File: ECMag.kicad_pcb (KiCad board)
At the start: 2 copper layers, 48 parts, among them J1 Conn_01x12, J2 Conn_01x05, J3 Conn_01x04, J4 USB_B, J5 Barrel_Jack_SW, J6 Conn_01x04, K1 Tactil Switch NA, K2 Tactil Switch B3F NA, K3 Tactil Switch NA, K4 Tactil Switch NA, P1 25K, Q1 BC548, U1 ATmega328P-PU, U2 PIC18F2550-ISO, U3 LM2577, Y1 16MHz, Y2 20MHz

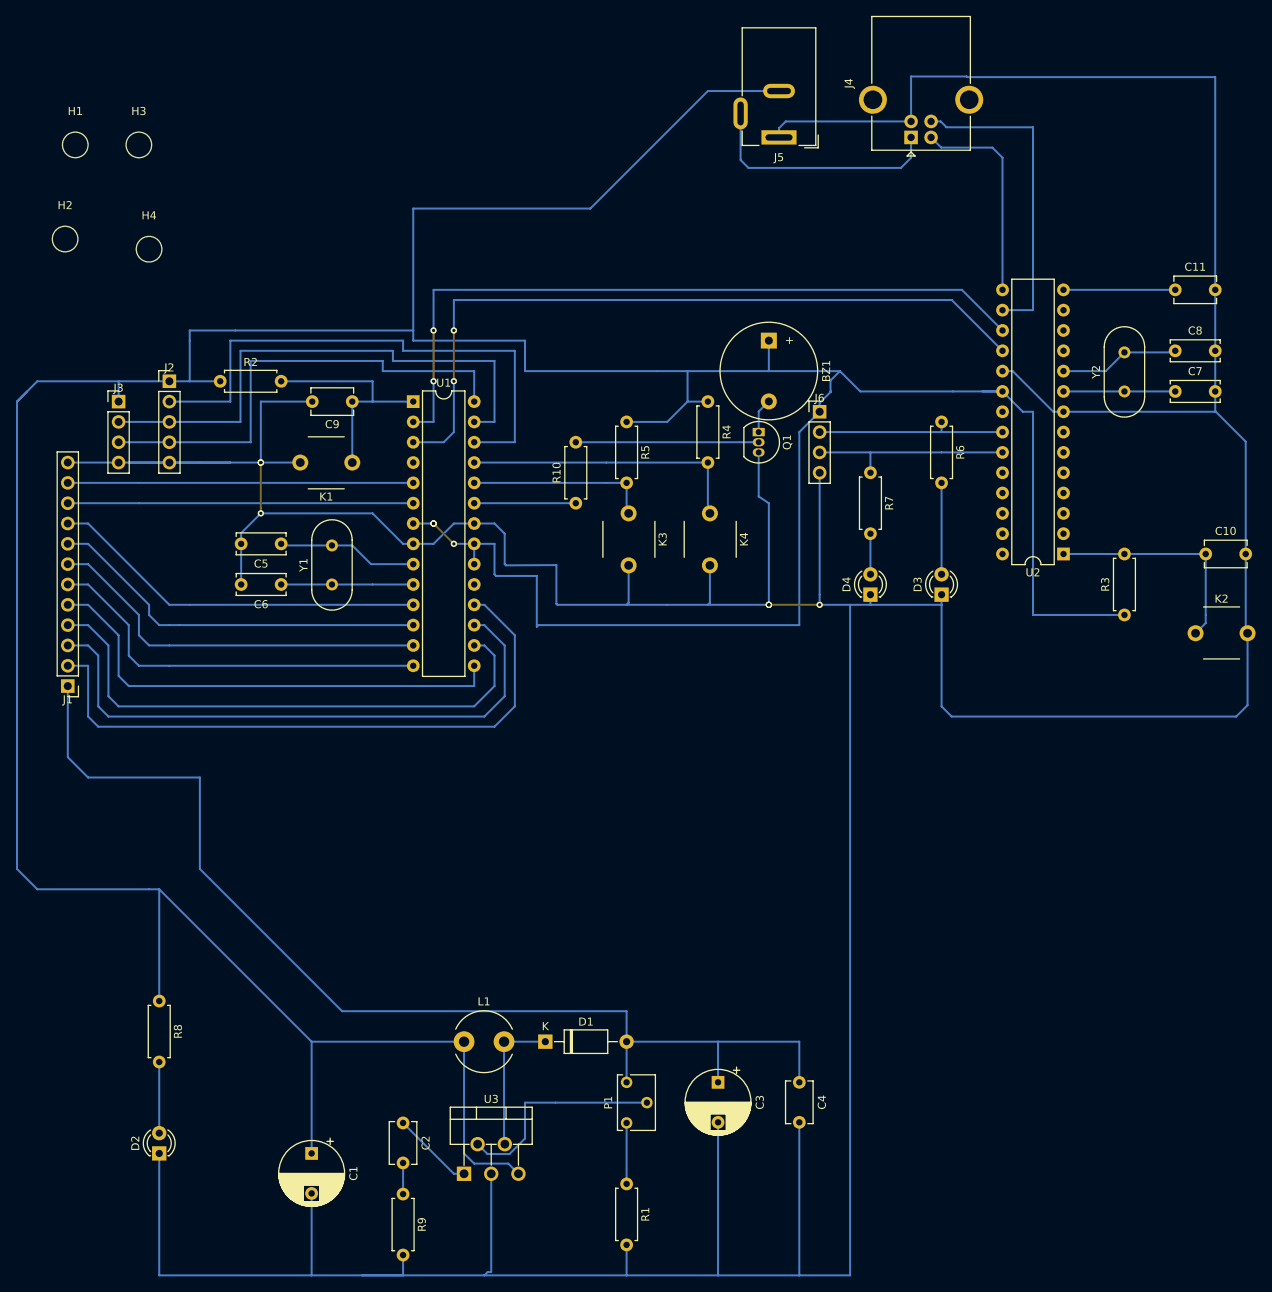
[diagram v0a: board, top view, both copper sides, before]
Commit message: primera versión del pcb
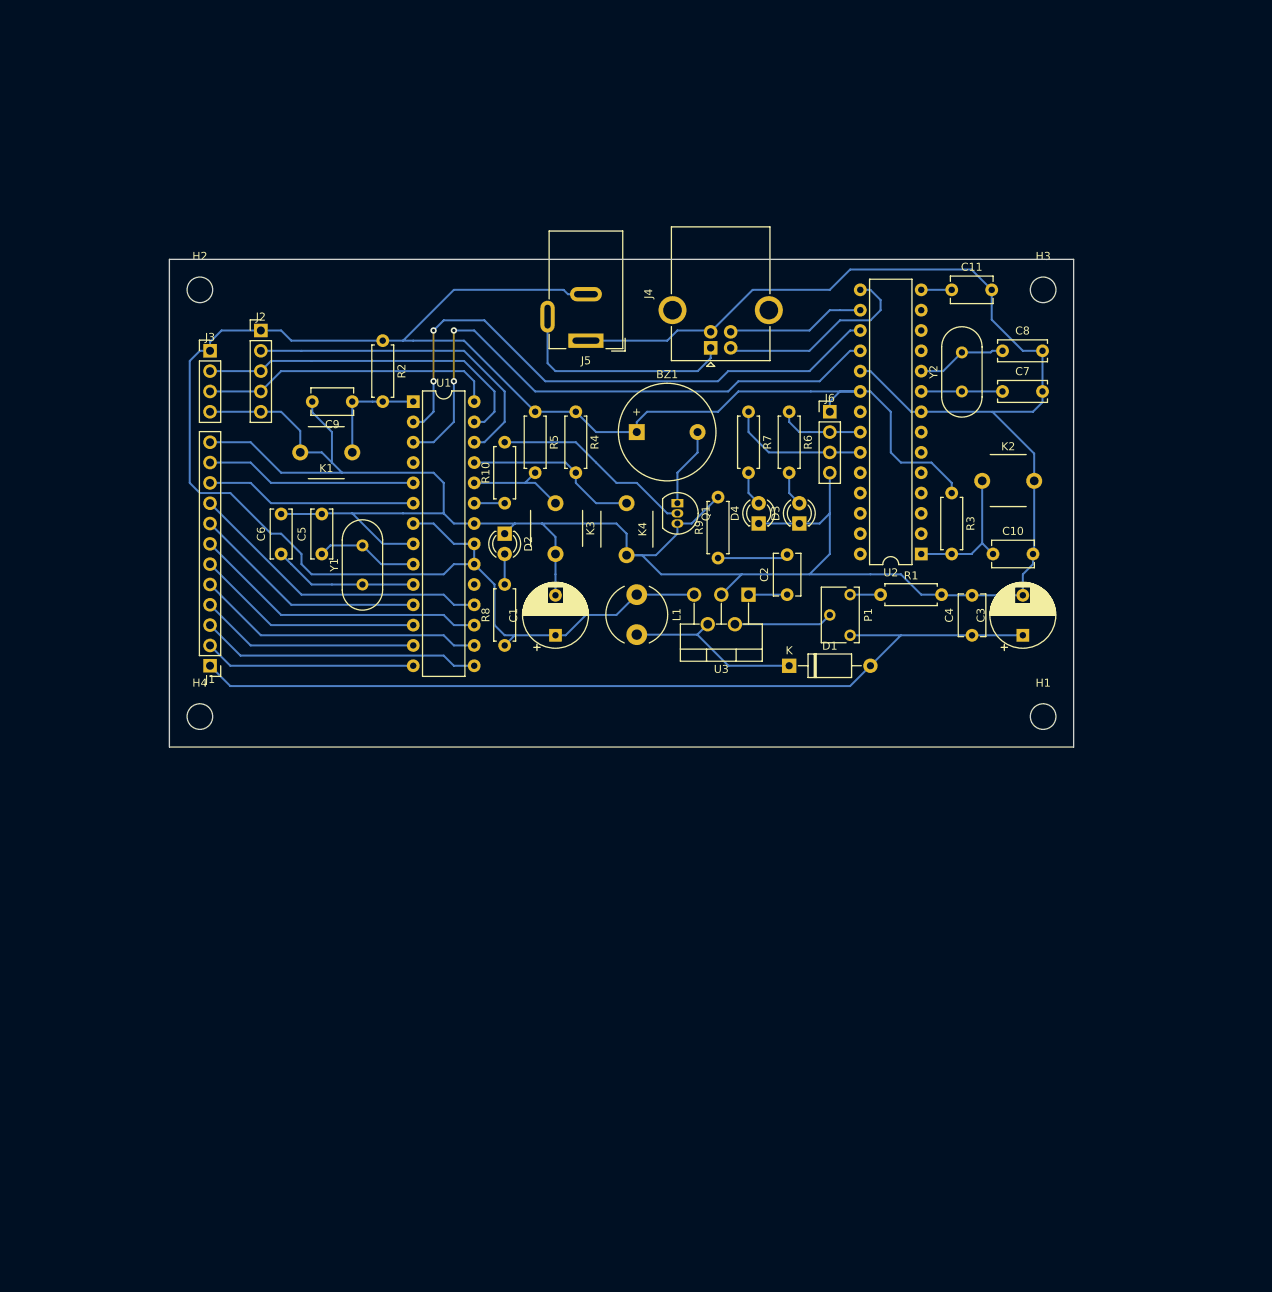
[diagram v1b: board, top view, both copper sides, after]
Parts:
- K1, K3, K4: value Tactil Switch NA -> Tactil Switch B3F NA
- K2: value Tactil Switch B3F NA -> Switch B3F NA
- U1: value ATmega328P-PU -> ATMega328
- U2: value PIC18F2550-ISO -> PIC18F2550
- moved H1 140.5 mm to (193.0, 106.7)
- moved H3 114.5 mm to (193.0, 53.3)
- moved R9 88.7 mm to (152.4, 86.9), turned to 90 degrees
- moved D2 88.7 mm to (125.7, 83.8), turned to 270 degrees
- moved C2 81.6 mm to (161.0, 91.4), turned to 90 degrees
- moved U3 80.7 mm to (156.2, 91.4), turned to 180 degrees
- moved R1 80.2 mm to (172.7, 91.4), turned to 0 degrees
- moved C1 71.6 mm to (132.1, 96.5), turned to 90 degrees
- moved C3 67.6 mm to (190.5, 96.5), turned to 90 degrees
- moved P1 62.5 mm to (168.9, 96.5), turned to 270 degrees
- moved R8 62.0 mm to (125.7, 97.8), turned to 90 degrees
- moved C4 59.9 mm to (184.2, 96.5), turned to 90 degrees
- moved L1 59.9 mm to (142.2, 91.4), turned to 270 degrees
- moved H4 58.8 mm to (87.6, 106.7)
- moved D1 56.0 mm to (161.3, 100.3)
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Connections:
- U1 pad 11: /a8 -> /a7
- U1 pad 12: /a7 -> /a5
- U1 pad 13: /a6 -> /a3
- U1 pad 14: /a5 -> /a1
- U1 pad 15: /a4 -> /a2
- U1 pad 16: /a3 -> /a4
- U1 pad 17: /a2 -> /a6
- U1 pad 18: /a1 -> /a8
- U1 pad 19: Net-(U1-Pad19) -> (no net)
- U1 pad 4: Net-(U1-Pad4) -> (no net)
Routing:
- net GND: track 699.5 -> 351.0 mm, vias 6 -> 0
- net +5V: track 544.1 -> 253.2 mm, vias 3 -> 0
- net /a1: track 79.4 -> 26.5 mm
- net /a3: track 69.2 -> 27.5 mm
- net /a2: track 74.3 -> 35.1 mm
- net +12V: track 139.2 -> 111.6 mm
- net /DRDY: track 68.6 -> 41.3 mm
- net /a4: track 60.5 -> 36.2 mm
- net /SDA: track 67.3 -> 43.3 mm
- net /SCL: track 59.7 -> 37.1 mm
- net /D+: track 39.7 -> 17.3 mm
- net /a5: track 49.6 -> 28.6 mm
- net /TxRx: track 93.3 -> 73.6 mm
- net /RxTx: track 92.3 -> 72.9 mm
- net /a7: track 48.1 -> 29.6 mm
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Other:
- board outline added: 113 x 61 mm
